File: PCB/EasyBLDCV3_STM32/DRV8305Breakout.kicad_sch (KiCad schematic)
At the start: 16 parts, among them U2 IAUC60N04S6N031HATMA1, U3 2EDL05N06PF

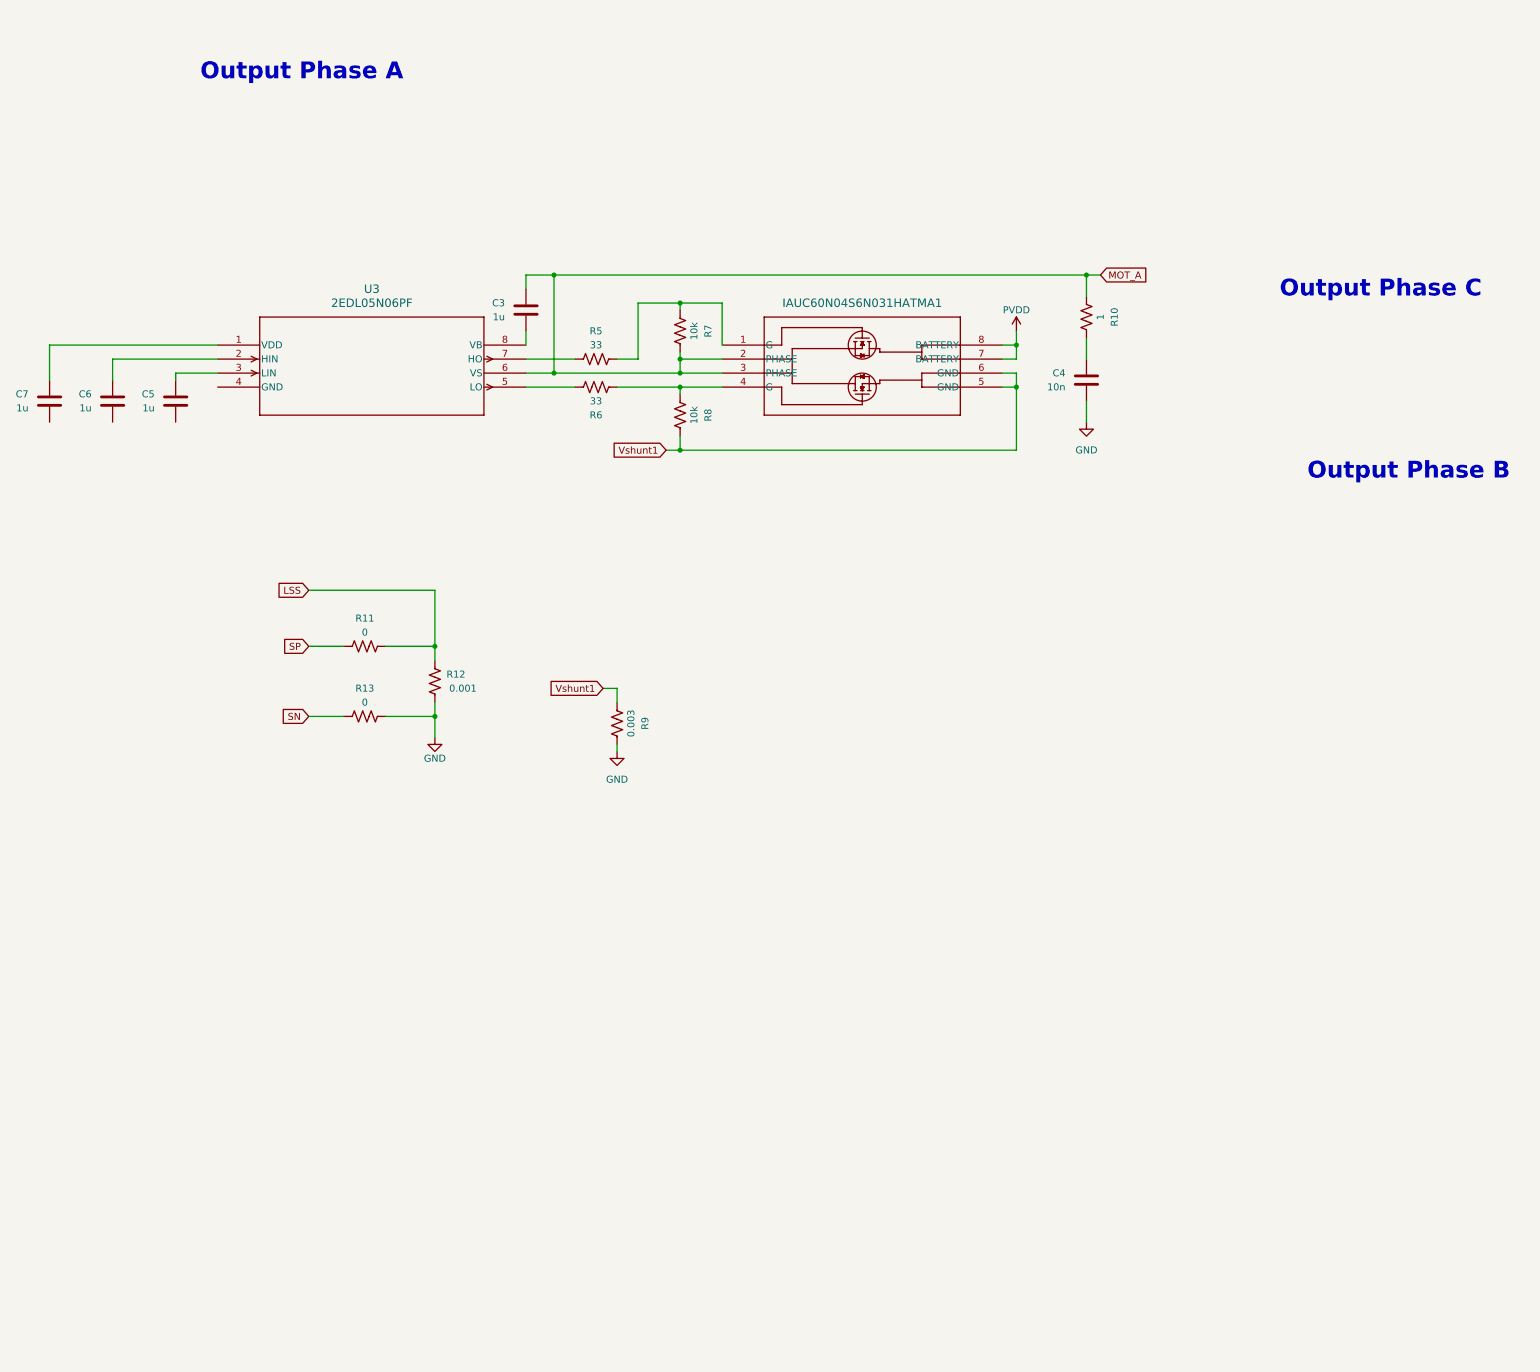
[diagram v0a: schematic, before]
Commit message: Created V4 Project
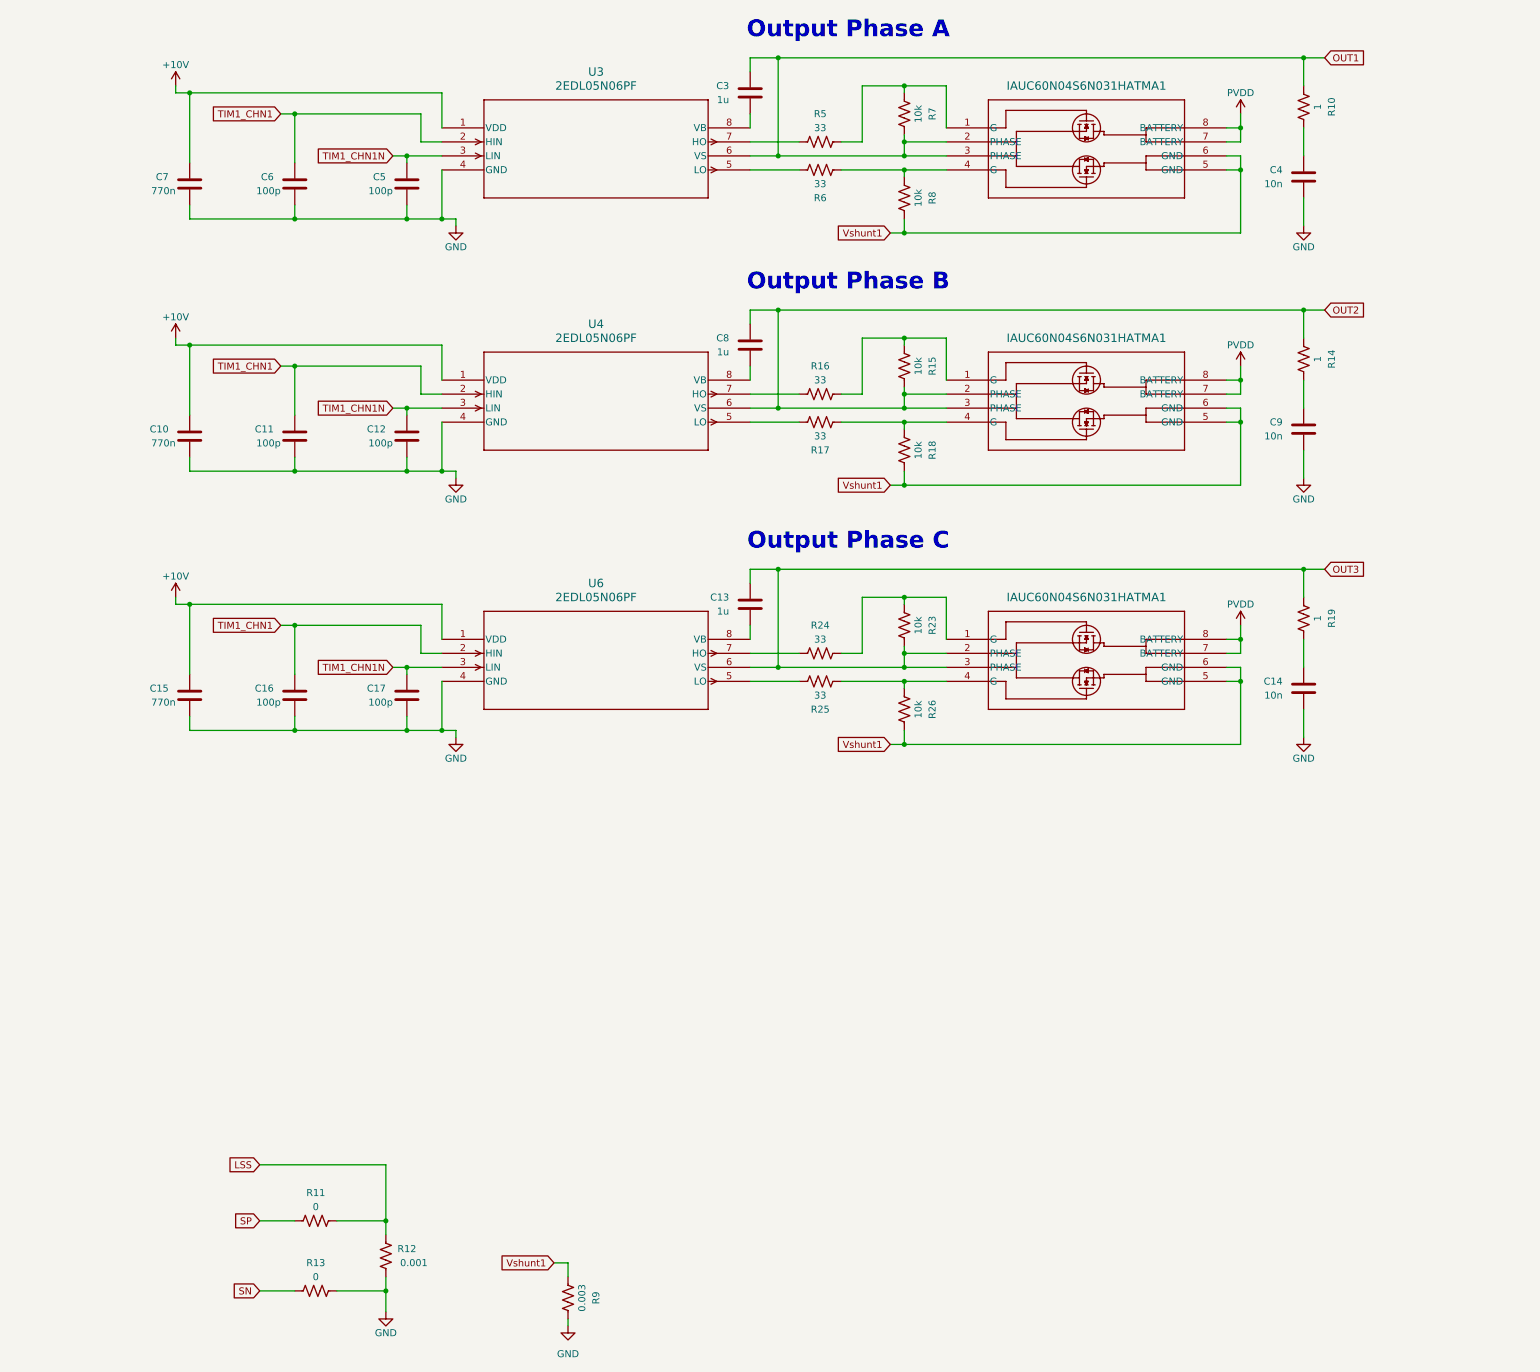
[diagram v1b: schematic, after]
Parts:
- added C10, C15: 770n, symbol Device:C
- added C11, C12, C16, C17: 100p, symbol Device:C
- added C13, C8: 1u, symbol Device:C
- added C14, C9: 10n, symbol Device:C
- added R14, R19: 1, Resistor_SMD:R_0603_1608Metric, symbol Device:R_US
- added R15, R18, R23, R26: 10k, Resistor_SMD:R_0603_1608Metric, symbol Device:R_US
- added R16, R17, R24, R25: 33, Resistor_SMD:R_0603_1608Metric, symbol Device:R_US
- added U4, U6: 2EDL05N06PF, PG-DSO-8-1_INF, symbol EasyBLDC:2EDL05N06PF
- added U5, U7: IAUC60N04S6N031HATMA1, PG-TDSON-8-56, symbol EasyBLDC:IAUC60N04S6N031HATMA1
- C5, C6: value 1u -> 100p
- C7: value 1u -> 770n
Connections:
- net GND: now also C5.1, C6.1, C7.1, U3.4 (GND), C10.1, C11.1, C12.1, C14.1, C15.1, C16.1, C17.1, C9.1, U4.4 (GND), U6.4 (GND)
- net PVDD: now also U5.7 (BATTERY), U5.8 (BATTERY), U7.7 (BATTERY), U7.8 (BATTERY)
- net Vshunt1: now also R18.1, R26.1, U5.5 (GND), U5.6 (GND), U7.5 (GND), U7.6 (GND)
- net TIM1_CHN1N: now reaches C5.2, U3.3 (LIN)
- net TIM1_CHN1N: now also C12.2, C17.2, U4.3 (LIN), U6.3 (LIN)
- net +10V: now reaches C7.2, U3.1 (VDD)
- net +10V: now also C10.2, C15.2, U4.1 (VDD), U6.1 (VDD)
- net TIM1_CHN1: now reaches C6.2, U3.2 (HIN)
- net TIM1_CHN1: now also C11.2, C16.2, U4.2 (HIN), U6.2 (HIN)
- net MOT_A renamed OUT1
- new net: C9.2, R14.1
- new net: C13.1, U6.8 (VB)
- new net: C14.2, R19.1
- new net: R17.1, U4.5 (LO)
- new net: R17.2, R18.2, U5.4 (G)
- new net: R23.2, R24.1, U7.1 (G)
- new net: R15.2, R16.1, U5.1 (G)
- new net: R16.2, U4.7 (HO)
- new net: R25.2, R26.2, U7.4 (G)
- new net: C8.1, U4.8 (VB)
- new net: R25.1, U6.5 (LO)
- new net: R24.2, U6.7 (HO)
- new net OUT2: C8.2, R14.2, R15.1, U4.6 (VS), U5.2 (PHASE), U5.3 (PHASE)
- new net OUT3: C13.2, R19.2, R23.1, U6.6 (VS), U7.2 (PHASE), U7.3 (PHASE)
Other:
- moved on the sheet: C3, C4, C5, C6, C7, R10, R11, R12, R13, R5, R6, R7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
